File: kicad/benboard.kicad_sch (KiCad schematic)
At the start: 63 parts, among them J1 USB_C_Receptacle_USB2.0, J3 Conn_ARM_SWD_TagConnect_TC203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, J4 Conn_01x02_Pin, J5 Conn_Coaxial, SW1 SW_Push, SW22 SW_Push, U1 nRF52840, U2 BQ24075RGT, Y1 32MHz, Y2 32.768kHz

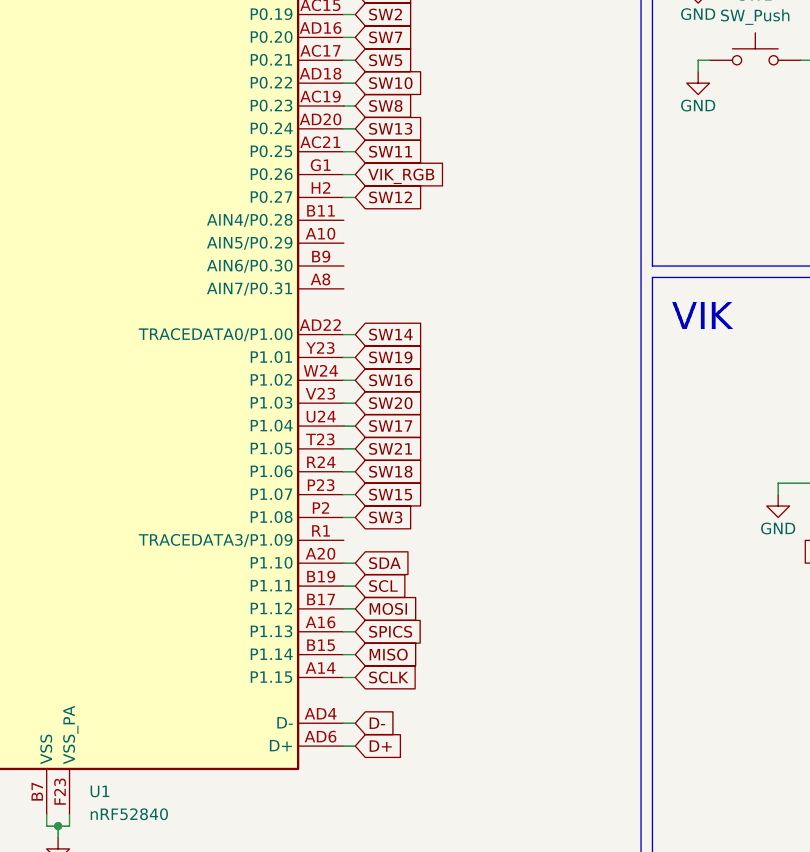
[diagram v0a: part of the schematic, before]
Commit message: VIK Compatible
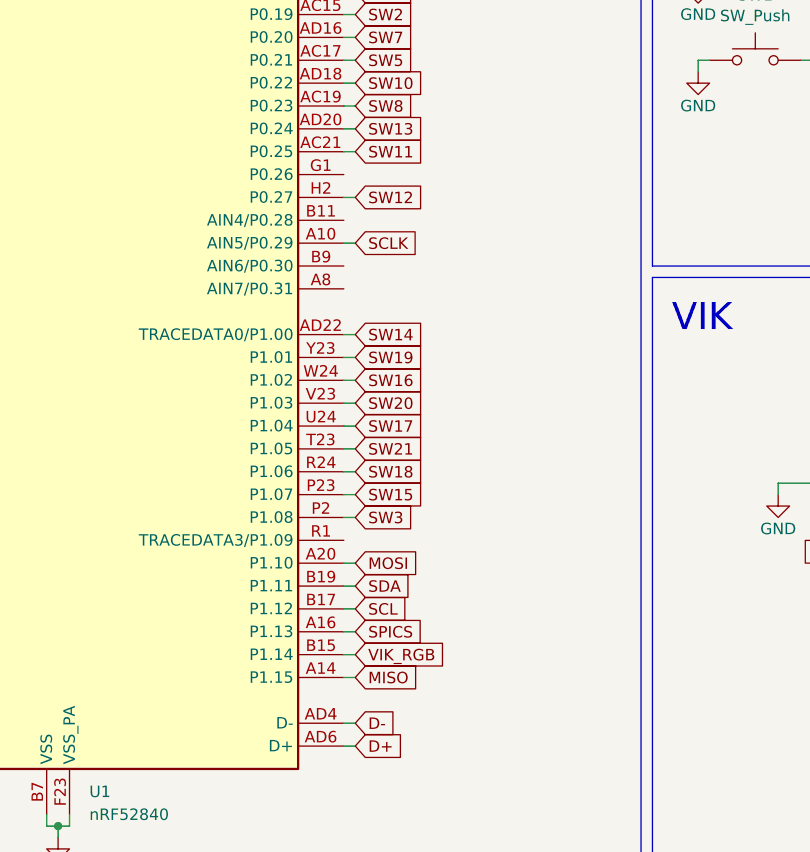
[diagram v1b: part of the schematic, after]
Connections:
- net MISO: now also U1.A14 (P1.15); no longer U1.B15 (P1.14)
- net MOSI: now also U1.A20 (P1.10); no longer U1.B17 (P1.12)
- net SCL: now also U1.B17 (P1.12); no longer U1.B19 (P1.11)
- net SCLK: now also U1.A10 (AIN5/P0.29); no longer U1.A14 (P1.15)
- net SDA: now also U1.B19 (P1.11); no longer U1.A20 (P1.10)
- net VIK_RGB: now also U1.B15 (P1.14); no longer U1.G1 (P0.26)

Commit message: proper footprint
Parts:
- J5: footprint Connector_Coaxial:SMA_Amphenol_132134-10_Vertical -> Connector_Coaxial:U.FL_Hirose_U.FL-R-SMT-1_Vertical
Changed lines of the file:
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@@
       (effects (font (size 1.27 1.27)))
     )
-    (property "Footprint" "Connector_Coaxial:SMA_Amphenol_132134-10_Vertical" (at 27.94 102.87 0)
+    (property "Footprint" "Connector_Coaxial:U.FL_Hirose_U.FL-R-SMT-1_Vertical" (at 27.94 102.87 0)
       (effects (font (size 1.27 1.27)) hide)
     )
